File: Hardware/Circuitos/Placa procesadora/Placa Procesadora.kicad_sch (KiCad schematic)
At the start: 6 parts, among them J1 Conn_01x02

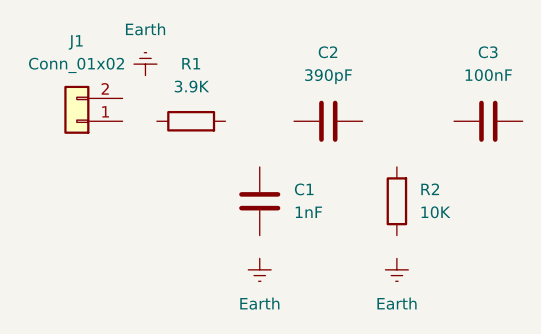
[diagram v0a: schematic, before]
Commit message: Placa procesadora - Conexión de filtros
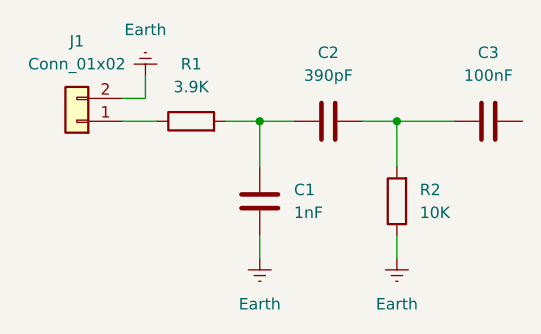
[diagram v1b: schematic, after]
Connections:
- net Earth: now also C1.2, J1.2 (Pin_2), R2.1
- net at C1.1: now also C2.1, R1.2
- net at C2.2: now also C3.1, R2.2
- net at R1.1: now also J1.1 (Pin_1)
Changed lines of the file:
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@@
 	(generator_version "10.0")
 	(paper "A4")
+	(junction
+		(at 77.47 73.66)
+		(diameter 0)
+		(color 0 0 0 0)
+	)
+	(junction
+		(at 62.23 73.66)
+		(diameter 0)
+		(color 0 0 0 0)
+	)
+	(wire
+		(pts
+			(xy 62.23 73.66) (xy 66.04 73.66)
+		)
+		(stroke
+			(width 0)
+			(type default)
+		)
+	)
+	(wire
+		(pts
+			(xy 49.53 68.58) (xy 49.53 71.12)
+		)
+		(stroke
+			(width 0)
+			(type default)
+		)
+	)
+	(wire
+		(pts
+			(xy 77.47 86.36) (xy 77.47 88.9)
+		)
+		(stroke
+			(width 0)
+			(type default)
+		)
+	)
+	(wire
+		(pts
+			(xy 49.53 71.12) (xy 46.99 71.12)
+		)
+		(stroke
+			(width 0)
+			(type default)
+		)
+	)
+	(wire
+		(pts
+			(xy 77.47 73.66) (xy 83.82 73.66)
+		)
+		(stroke
+			(width 0)
+			(type default)
+		)
+	)
+	(wire
+		(pts
+			(xy 58.42 73.66) (xy 62.23 73.66)
+		)
+		(stroke
+			(width 0)
+			(type default)
+		)
+	)
+	(wire
+		(pts
+			(xy 73.66 73.66) (xy 77.47 73.66)
+		)
+		(stroke
+			(width 0)
+			(type default)
+		)
+	)
+	(wire
+		(pts
+			(xy 62.23 86.36) (xy 62.23 88.9)
+		)
+		(stroke
+			(width 0)
+			(type default)
+		)
+	)
+	(wire
+		(pts
+			(xy 62.23 73.66) (xy 62.23 78.74)
+		)
+		(stroke
+			(width 0)
+			(type default)
+		)
+	)
+	(wire
+		(pts
+			(xy 46.99 73.66) (xy 50.8 73.66)
+		)
+		(stroke
+			(width 0)
+			(type default)
+		)
+	)
+	(wire
+		(pts
+			(xy 77.47 73.66) (xy 77.47 78.74)
+		)
+		(stroke
+			(width 0)
+			(type default)
+		)
+	)
 	(symbol
 		(lib_id "Device:C")
